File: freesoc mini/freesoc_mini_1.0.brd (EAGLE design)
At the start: 50.8 x 17.8 mm, 50 parts, among them IC1 CY7C68013A-56QFNLFXC, IC2 24LC00OT, Y1 XRCGB24M000F0L00R0

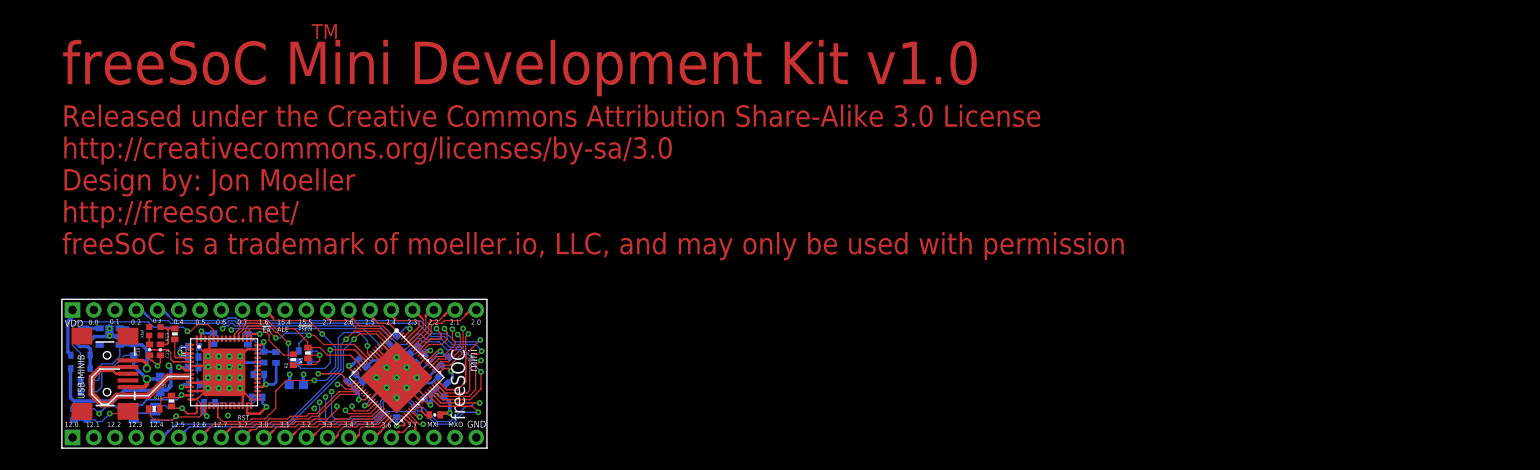
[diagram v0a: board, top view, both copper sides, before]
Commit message: Updates to boards for production
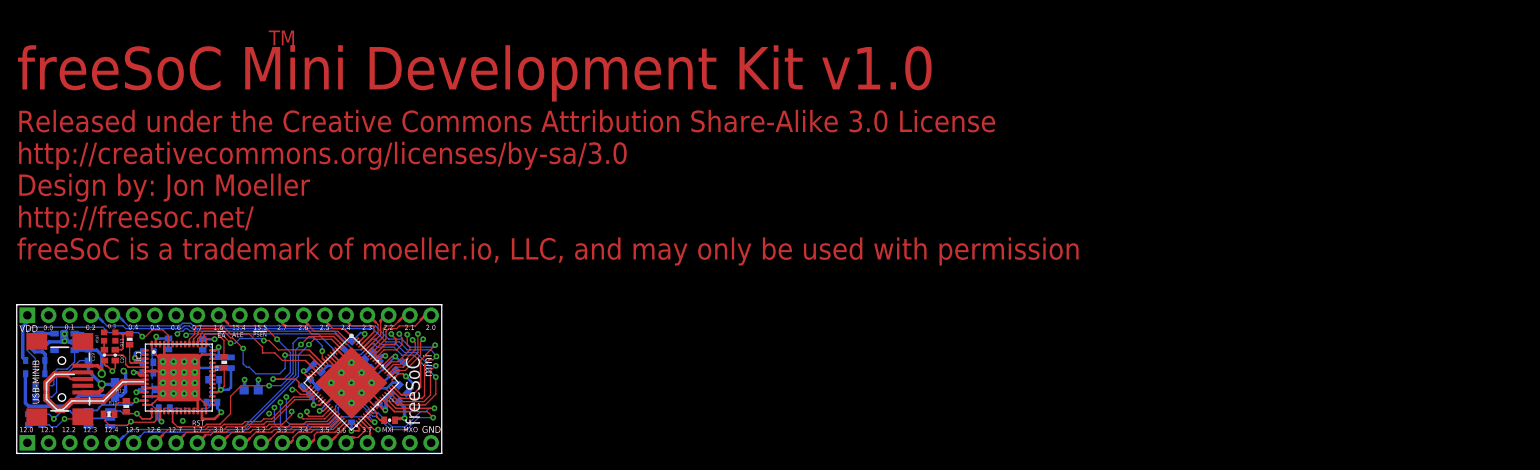
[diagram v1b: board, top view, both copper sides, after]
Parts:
- removed R3, R4, R5: NOLOAD, SparkFun:0402-RES
- moved R8 8.26 mm to (24.8, 10.9)
- moved C1 5.43 mm to (24.1, 10.9)
- moved C11 5.43 mm to (39.6, 13.0)
- moved C12 5.43 mm to (35.5, 7.45)
- moved C13 5.43 mm to (42.1, 11.8)
- moved C14 5.43 mm to (45.8, 10.4)
- moved C15 5.43 mm to (40.0, 4.37)
- moved C19 5.43 mm to (10.5, 11.7)
- moved C2 5.43 mm to (15.7, 12.1)
- moved C21 5.43 mm to (15.7, 9.64)
- moved C22 5.43 mm to (17.6, 5.42)
- moved C24 5.43 mm to (23.5, 8.81)
- moved C25 5.43 mm to (18.1, 13.1)
- moved C26 5.43 mm to (15.8, 7.64)
- moved C29 5.43 mm to (8.57, 11.7)
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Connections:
- net SWDCK: no longer R4.1
- net SWDIO: no longer R3.1
- net SWV: no longer R5.1
- net VCC: no longer R3.2, R4.2, R5.2
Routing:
- net VCC: track 70.7 -> 63.1 mm, vias 11 -> 10
- net SWDIO: track 21.0 -> 18.2 mm
- net N$2: track 8.26 -> 5.91 mm
- net SWDCK: track 23.2 -> 22.2 mm
- net VDD: track 68.9 -> 69.8 mm
- net GND: track 125.2 -> 125.9 mm
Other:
- board text added: "freeSoC"
- board text removed: "freeSOC"
